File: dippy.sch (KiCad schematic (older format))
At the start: 12 parts, among them J1 Conn_01x02_Female, U1 ATmega328P-PU, U2 RFM95W-915S2, U3 MCP1700-3302E_SOT23, Y1 Crystal_GND2

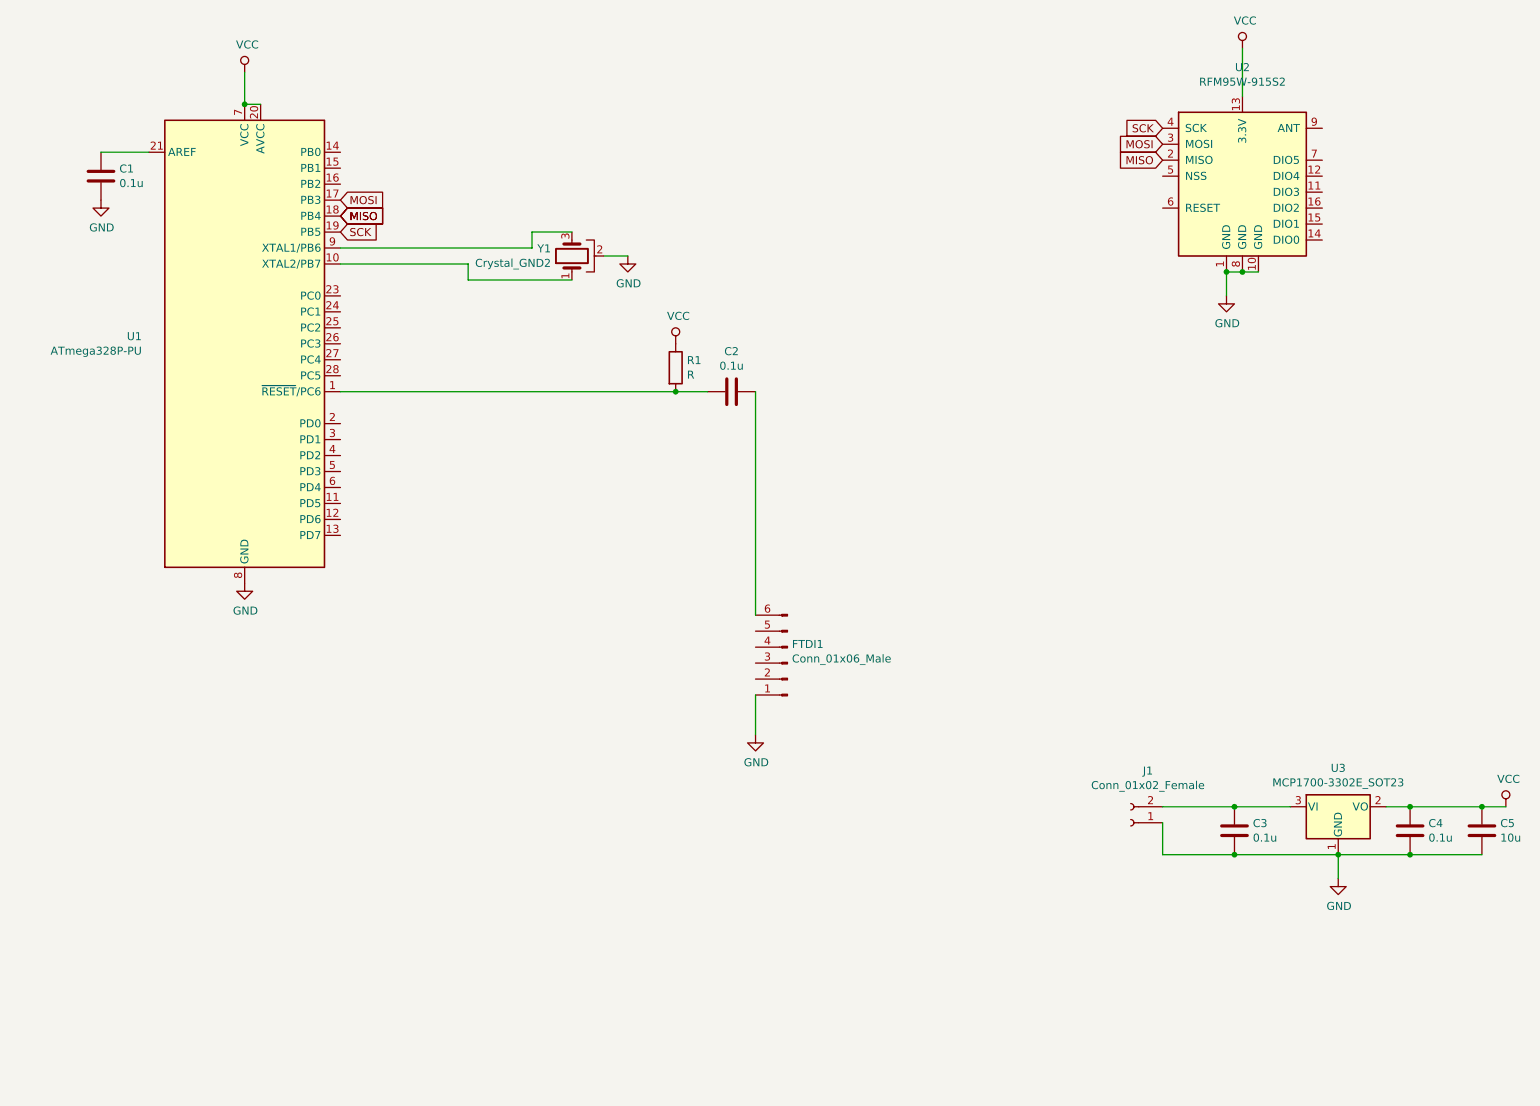
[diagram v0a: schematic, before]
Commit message: update
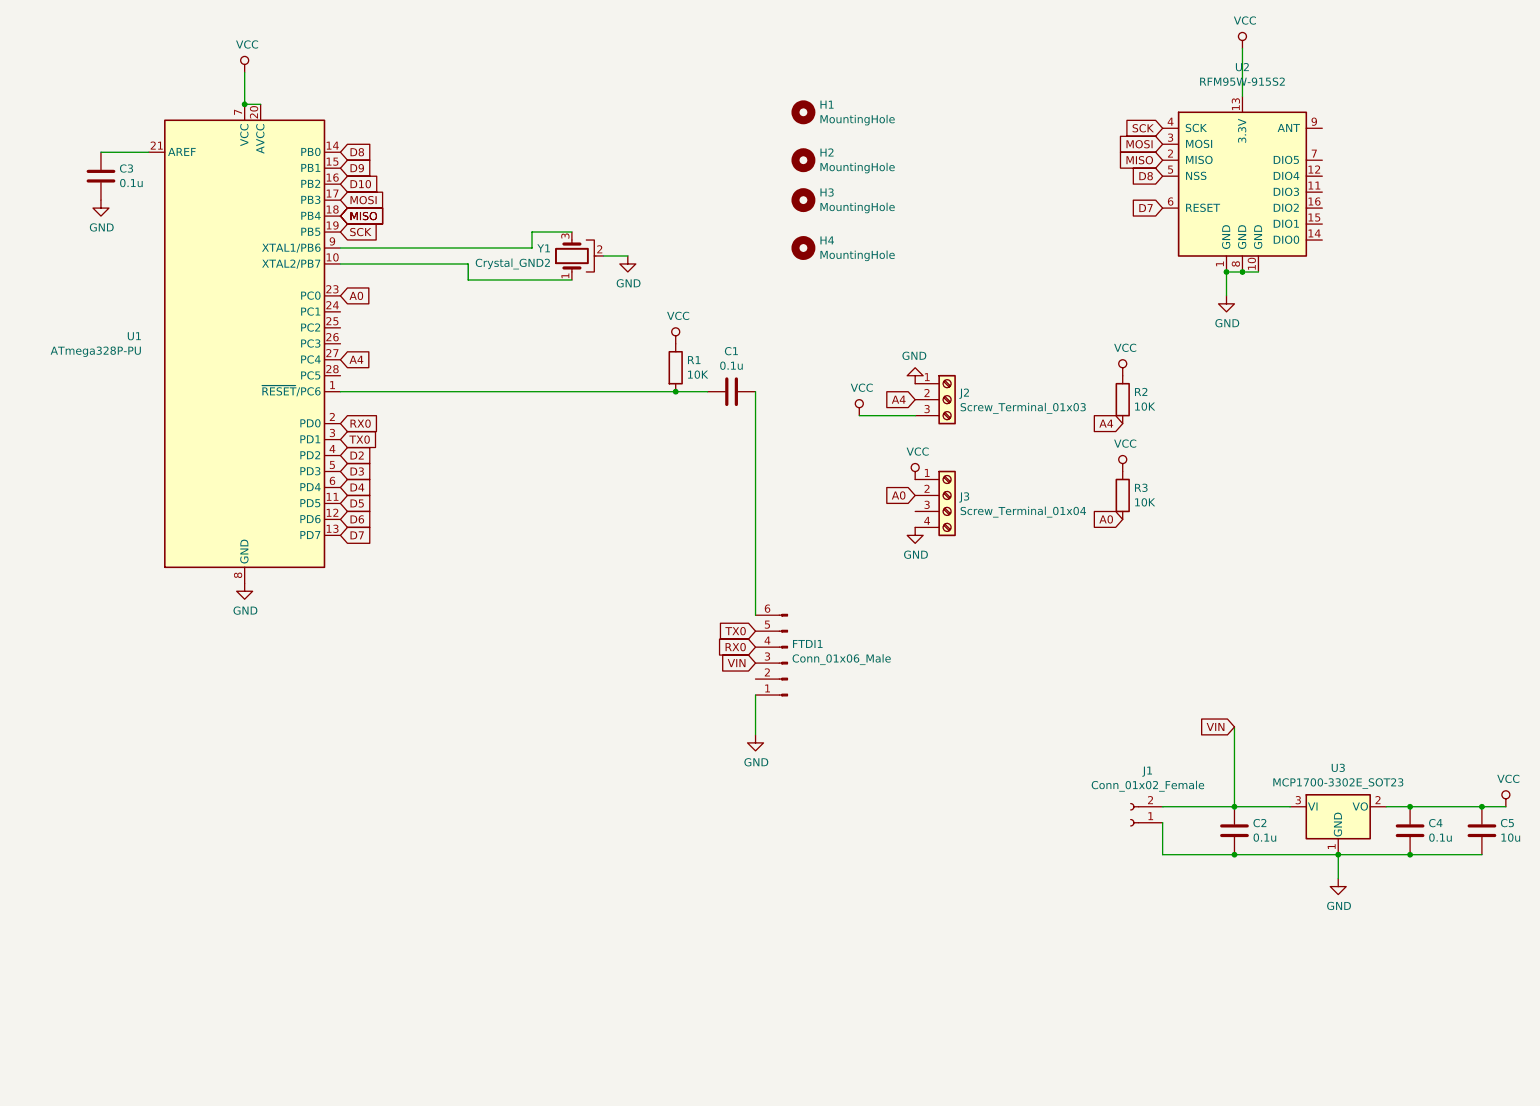
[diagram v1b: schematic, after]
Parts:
- added H1, H2, H3, H4: MountingHole, MountingHole:MountingHole_2.7mm_M2.5, symbol Mechanical:MountingHole
- added J2: Screw_Terminal_01x03, TerminalBlock_Phoenix:TerminalBlock_Phoenix_PT-1,5-3-3.5-H_1x03_P3.50mm_Horizontal, symbol Connector:Screw_Terminal_01x03
- added J3: Screw_Terminal_01x04, TerminalBlock_Phoenix:TerminalBlock_Phoenix_PT-1,5-4-3.5-H_1x04_P3.50mm_Horizontal, symbol Connector:Screw_Terminal_01x04
- added R2, R3: 10K, Resistor_THT:R_Axial_DIN0207_L6.3mm_D2.5mm_P2.54mm_Vertical, symbol Device:R
- C1: renamed from C2; footprint (none) -> Capacitor_THT:C_Disc_D3.0mm_W1.6mm_P2.50mm
- C2: renamed from C3; footprint (none) -> Capacitor_THT:C_Disc_D3.0mm_W1.6mm_P2.50mm
- C3: renamed from C1; footprint (none) -> Capacitor_THT:C_Disc_D3.0mm_W1.6mm_P2.50mm
- C4: footprint (none) -> Capacitor_THT:C_Disc_D3.0mm_W1.6mm_P2.50mm
- C5: footprint (none) -> Capacitor_THT:CP_Radial_D5.0mm_P2.50mm
- FTDI1: footprint (none) -> Connector_PinHeader_2.54mm:PinHeader_1x06_P2.54mm_Horizontal
- J1: footprint (none) -> Connector_PinSocket_2.54mm:PinSocket_1x02_P2.54mm_Vertical
- R1: value R -> 10K; footprint (none) -> Resistor_THT:R_Axial_DIN0207_L6.3mm_D2.5mm_P2.54mm_Vertical
- U3: footprint Package_TO_SOT_SMD:SOT-23 -> Package_TO_SOT_THT:TO-92L_Wide
- Y1: footprint (none) -> Connector_PinSocket_2.54mm:PinSocket_1x03_P2.54mm_Vertical
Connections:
- net GND: now also J2.1 (Pin_1), J3.4 (Pin_4)
- net VCC: now also J2.3 (Pin_3), J3.1 (Pin_1), R2.1, R3.1
- net D5: now reaches U1.11 (PD5)
- net D6: now reaches U1.12 (PD6)
- net D7: now reaches U1.13 (PD7)
- net D7: now also U2.6 (RESET)
- net D8: now reaches U1.14 (PB0)
- net D8: now also U2.5 (NSS)
- net D9: now reaches U1.15 (PB1)
- net D10: now reaches U1.16 (PB2)
- net RX0: now reaches U1.2 (PD0)
- net RX0: now also FTDI1.4 (Pin_4)
- net A0: now reaches U1.23 (PC0)
- net A0: now also J3.2 (Pin_2), R3.2
- net A4: now reaches U1.27 (PC4)
- net A4: now also J2.2 (Pin_2), R2.2
- net TX0: now reaches U1.3 (PD1)
- net TX0: now also FTDI1.5 (Pin_5)
- net D2: now reaches U1.4 (PD2)
- net D3: now reaches U1.5 (PD3)
- net D4: now reaches U1.6 (PD4)
- net VIN: now reaches FTDI1.3 (Pin_3)
- net VIN: now also C2.1, J1.2 (Pin_2), U3.3 (VI)
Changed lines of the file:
@@
 F 0 "Y1" V 4796 2231 50  0000 L CNN
 F 1 "Crystal_GND2" V 4705 2231 50  0000 L CNN
-F 2 "" H 4750 2100 50  0001 C CNN
+F 2 "Connector_PinSocket_2.54mm:PinSocket_1x03_P2.54mm_Vertical" H 4750 2100 50  0001 C CNN
 F 3 "~" H 4750 2100 50  0001 C CNN
 	1    4750 2100
@@
 P 5400 2800
 F 0 "R1" H 5470 2846 50  0000 L CNN
-F 1 "R" H 5470 2755 50  0000 L CNN
-F 2 "" V 5330 2800 50  0001 C CNN
+F 1 "10K" H 5470 2755 50  0000 L CNN
+F 2 "Resistor_THT:R_Axial_DIN0207_L6.3mm_D2.5mm_P2.54mm_Vertical" V 5330 2800 50  0001 C CNN
 F 3 "~" H 5400 2800 50  0001 C CNN
 	1    5400 2800
@@
 $EndComp
 $Comp
-L Device:C C1
+L Device:C C3
 U 1 1 5F266C1D
 P 1800 1600
-F 0 "C1" H 1915 1646 50  0000 L CNN
+F 0 "C3" H 1915 1646 50  0000 L CNN
 F 1 "0.1u" H 1915 1555 50  0000 L CNN
-F 2 "" H 1838 1450 50  0001 C CNN
+F 2 "Capacitor_THT:C_Disc_D3.0mm_W1.6mm_P2.50mm" H 1838 1450 50  0001 C CNN
 F 3 "~" H 1800 1600 50  0001 C CNN
 	1    1800 1600
@@
 $EndComp
 $Comp
-L Device:C C2
+L Device:C C1
 U 1 1 5F26DE4A
 P 5750 2950
-F 0 "C2" V 5498 2950 50  0000 C CNN
+F 0 "C1" V 5498 2950 50  0000 C CNN
 F 1 "0.1u" V 5589 2950 50  0000 C CNN
-F 2 "" H 5788 2800 50  0001 C CNN
+F 2 "Capacitor_THT:C_Disc_D3.0mm_W1.6mm_P2.50mm" H 5788 2800 50  0001 C CNN
 F 3 "~" H 5750 2950 50  0001 C CNN
 	1    5750 2950
@@
 F 0 "U3" H 9550 5792 50  0000 C CNN
 F 1 "MCP1700-3302E_SOT23" H 9550 5701 50  0000 C CNN
-F 2 "Package_TO_SOT_SMD:SOT-23" H 9550 5775 50  0001 C CNN
+F 2 "Package_TO_SOT_THT:TO-92L_Wide" H 9550 5775 50  0001 C CNN
 F 3 "http://ww1.microchip.com/downloads/en/DeviceDoc/20001826D.pdf" H 9550 5550 50  0001 C CNN
 	1    9550 5550
@@
 F 0 "J1" H 8142 5325 50  0000 C CNN
 F 1 "Conn_01x02_Female" H 8142 5416 50  0000 C CNN
-F 2 "" H 8250 5650 50  0001 C CNN
+F 2 "Connector_PinSocket_2.54mm:PinSocket_1x02_P2.54mm_Vertical" H 8250 5650 50  0001 C CNN
 F 3 "~" H 8250 5650 50  0001 C CNN
 	1    8250 5650
@@
 	8450 5650 8450 5850
 $Comp
-L Device:C C3
+L Device:C C2
 U 1 1 5F27AAEF
 P 8900 5700
-F 0 "C3" H 9015 5746 50  0000 L CNN
+F 0 "C2" H 9015 5746 50  0000 L CNN
 F 1 "0.1u" H 9015 5655 50  0000 L CNN
-F 2 "" H 8938 5550 50  0001 C CNN
+F 2 "Capacitor_THT:C_Disc_D3.0mm_W1.6mm_P2.50mm" H 8938 5550 50  0001 C CNN
 F 3 "~" H 8900 5700 50  0001 C CNN
 	1    8900 5700
@@
 F 0 "C4" H 10115 5746 50  0000 L CNN
 F 1 "0.1u" H 10115 5655 50  0000 L CNN
-F 2 "" H 10038 5550 50  0001 C CNN
+F 2 "Capacitor_THT:C_Disc_D3.0mm_W1.6mm_P2.50mm" H 10038 5550 50  0001 C CNN
 F 3 "~" H 10000 5700 50  0001 C CNN
 	1    10000 5700
@@
 F 0 "C5" H 10565 5746 50  0000 L CNN
 F 1 "10u" H 10565 5655 50  0000 L CNN
-F 2 "" H 10488 5550 50  0001 C CNN
+F 2 "Capacitor_THT:CP_Radial_D5.0mm_P2.50mm" H 10488 5550 50  0001 C CNN
 F 3 "~" H 10450 5700 50  0001 C CNN
 	1    10450 5700
@@
 F 0 "FTDI1" H 6072 4532 50  0000 R CNN
 F 1 "Conn_01x06_Male" H 6072 4623 50  0000 R CNN
-F 2 "" H 6100 4650 50  0001 C CNN
+F 2 "Connector_PinHeader_2.54mm:PinHeader_1x06_P2.54mm_Horizontal" H 6100 4650 50  0001 C CNN
 F 3 "~" H 6100 4650 50  0001 C CNN
 	1    6100 4650
@@
 Wire Wire Line
 	3300 2150 4100 2150
+Text GLabel 3300 3450 2    50   Input ~ 0
+D3
+Text GLabel 3300 3550 2    50   Input ~ 0
+D4
+Text GLabel 3300 3650 2    50   Input ~ 0
+D5
+Text GLabel 3300 3750 2    50   Input ~ 0
+D6
+Text GLabel 5900 4650 0    50   Input ~ 0
+VIN
+Text GLabel 5900 4550 0    50   Input ~ 0
+RX0
+Text GLabel 5900 4450 0    50   Input ~ 0
+TX0
+Text GLabel 3300 3150 2    50   Input ~ 0
+RX0
+Text GLabel 3300 3250 2    50   Input ~ 0
+TX0
+Text GLabel 3300 3350 2    50   Input ~ 0
+D2
+Text GLabel 3300 3850 2    50   Input ~ 0
+D7
+Text GLabel 3300 1450 2    50   Input ~ 0
+D8
+Text GLabel 3300 1550 2    50   Input ~ 0
+D9
+Text GLabel 3300 1650 2    50   Input ~ 0
+D10
+Text GLabel 8450 1600 0    50   Input ~ 0
+D8
+Text GLabel 8450 1800 0    50   Input ~ 0
+D7
+$Comp
+L Mechanical:MountingHole H1
+U 1 1 5F2F7F92
+P 6200 1200
+F 0 "H1" H 6300 1246 50  0000 L CNN
+F 1 "MountingHole" H 6300 1155 50  0000 L CNN
+F 2 "MountingHole:MountingHole_2.7mm_M2.5" H 6200 1200 50  0001 C CNN
+F 3 "~" H 6200 1200 50  0001 C CNN
+	1    6200 1200
+	1    0    0    -1
+$EndComp
+$Comp
+L Mechanical:MountingHole H2
+U 1 1 5F2F84A7
+P 6200 1500
+F 0 "H2" H 6300 1546 50  0000 L CNN
+F 1 "MountingHole" H 6300 1455 50  0000 L CNN
+F 2 "MountingHole:MountingHole_2.7mm_M2.5" H 6200 1500 50  0001 C CNN
+F 3 "~" H 6200 1500 50  0001 C CNN
+	1    6200 1500
+	1    0    0    -1
+$EndComp
+$Comp
+L Mechanical:MountingHole H3
+U 1 1 5F30039A
+P 6200 1750
+F 0 "H3" H 6300 1796 50  0000 L CNN
+F 1 "MountingHole" H 6300 1705 50  0000 L CNN
+F 2 "MountingHole:MountingHole_2.7mm_M2.5" H 6200 1750 50  0001 C CNN
+F 3 "~" H 6200 1750 50  0001 C CNN
+	1    6200 1750
+	1    0    0    -1
+$EndComp
+$Comp
+L Mechanical:MountingHole H4
+U 1 1 5F30064C
+P 6200 2050
+F 0 "H4" H 6300 2096 50  0000 L CNN
+F 1 "MountingHole" H 6300 2005 50  0000 L CNN
+F 2 "MountingHole:MountingHole_2.7mm_M2.5" H 6200 2050 50  0001 C CNN
+F 3 "~" H 6200 2050 50  0001 C CNN
+	1    6200 2050
+	1    0    0    -1
+$EndComp
+$Comp
+L Connector:Screw_Terminal_01x03 J2
+U 1 1 5F31163E
+P 7100 3000
+F 0 "J2" H 7180 3042 50  0000 L CNN
+F 1 "Screw_Terminal_01x03" H 7180 2951 50  0000 L CNN
+F 2 "TerminalBlock_Phoenix:TerminalBlock_Phoenix_PT-1,5-3-3.5-H_1x03_P3.50mm_Horizontal" H 7100 3000 50  0001 C CNN
+F 3 "~" H 7100 3000 50  0001 C CNN
+	1    7100 3000
+	1    0    0    -1
+$EndComp
+$Comp
+L Connector:Screw_Terminal_01x04 J3
+U 1 1 5F312484
+P 7100 3600
+F 0 "J3" H 7180 3592 50  0000 L CNN
+F 1 "Screw_Terminal_01x04" H 7180 3501 50  0000 L CNN
+F 2 "TerminalBlock_Phoenix:TerminalBlock_Phoenix_PT-1,5-4-3.5-H_1x04_P3.50mm_Horizontal" H 7100 3600 50  0001 C CNN
+F 3 "~" H 7100 3600 50  0001 C CNN
+	1    7100 3600
+	1    0    0    -1
+$EndComp
+$Comp
+L power:VCC #PWR0111
+U 1 1 5F31DB78
+P 6550 3100
+F 0 "#PWR0111" H 6550 2950 50  0001 C CNN
+F 1 "VCC" H 6567 3273 50  0000 C CNN
+F 2 "" H 6550 3100 50  0001 C CNN
+F 3 "" H 6550 3100 50  0001 C CNN
+	1    6550 3100
+	1    0    0    -1
+$EndComp
+Wire Wire Line
+	6900 3100 6550 3100
+Text GLabel 3300 2750 2    50   Input ~ 0
+A4
+Text GLabel 6900 3000 0    50   Input ~ 0
+A4
+$Comp
+L power:GND #PWR0112
+U 1 1 5F3218C4
+P 6900 2900
+F 0 "#PWR0112" H 6900 2650 50  0001 C CNN
+F 1 "GND" H 6905 2727 50  0000 C CNN
+F 2 "" H 6900 2900 50  0001 C CNN
+F 3 "" H 6900 2900 50  0001 C CNN
+	1    6900 2900
+	-1   0    0    1
+$EndComp
+$Comp
+L Device:R R2
+U 1 1 5F322886
+P 8200 3000
+F 0 "R2" H 8270 3046 50  0000 L CNN
+F 1 "10K" H 8270 2955 50  0000 L CNN
+F 2 "Resistor_THT:R_Axial_DIN0207_L6.3mm_D2.5mm_P2.54mm_Vertical" V 8130 3000 50  0001 C CNN
+F 3 "~" H 8200 3000 50  0001 C CNN
+	1    8200 3000
+	1    0    0    -1
+$EndComp
+$Comp
+L power:VCC #PWR0113
+U 1 1 5F322DF7
+P 8200 2850
+F 0 "#PWR0113" H 8200 2700 50  0001 C CNN
+F 1 "VCC" H 8217 3023 50  0000 C CNN
+F 2 "" H 8200 2850 50  0001 C CNN
+F 3 "" H 8200 2850 50  0001 C CNN
+	1    8200 2850
+	1    0    0    -1
+$EndComp
+Text GLabel 8200 3150 0    50   Input ~ 0
+A4
+$Comp
+L power:VCC #PWR0114
+U 1 1 5F32A308
+P 6900 3500
+F 0 "#PWR0114" H 6900 3350 50  0001 C CNN
+F 1 "VCC" H 6917 3673 50  0000 C CNN
+F 2 "" H 6900 3500 50  0001 C CNN
+F 3 "" H 6900 3500 50  0001 C CNN
+	1    6900 3500
+	1    0    0    -1
+$EndComp
+Text GLabel 3300 2350 2    50   Input ~ 0
+A0
+Text GLabel 6900 3600 0    50   Input ~ 0
+A0
+$Comp
+L Device:R R3
+U 1 1 5F334BCF
+P 8200 3600
+F 0 "R3" H 8270 3646 50  0000 L CNN
+F 1 "10K" H 8270 3555 50  0000 L CNN
+F 2 "Resistor_THT:R_Axial_DIN0207_L6.3mm_D2.5mm_P2.54mm_Vertical" V 8130 3600 50  0001 C CNN
+F 3 "~" H 8200 3600 50  0001 C CNN
+	1    8200 3600
+	1    0    0    -1
+$EndComp
+$Comp
+L power:VCC #PWR0115
+U 1 1 5F3351C9
+P 8200 3450
+F 0 "#PWR0115" H 8200 3300 50  0001 C CNN
+F 1 "VCC" H 8217 3623 50  0000 C CNN
+F 2 "" H 8200 3450 50  0001 C CNN
+F 3 "" H 8200 3450 50  0001 C CNN
+	1    8200 3450
+	1    0    0    -1
+$EndComp
+Text GLabel 8200 3750 0    50   Input ~ 0
+A0
+$Comp
+L power:GND #PWR0116
+U 1 1 5F33656E
+P 6900 3800
+F 0 "#PWR0116" H 6900 3550 50  0001 C CNN
+F 1 "GND" H 6905 3627 50  0000 C CNN
+F 2 "" H 6900 3800 50  0001 C CNN
+F 3 "" H 6900 3800 50  0001 C CNN
+	1    6900 3800
+	1    0    0    -1
+$EndComp
+Text GLabel 8900 5050 0    50   Input ~ 0
+VIN
+Wire Wire Line
+	8900 5050 8900 5550
 $EndSCHEMATC

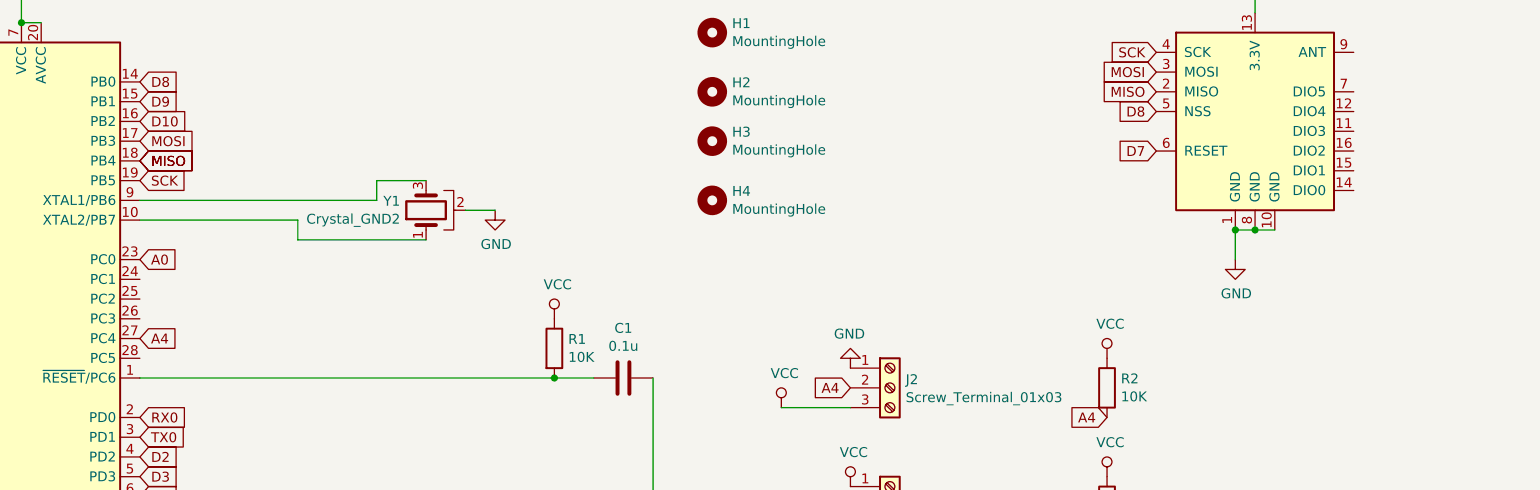
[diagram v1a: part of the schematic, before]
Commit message: update
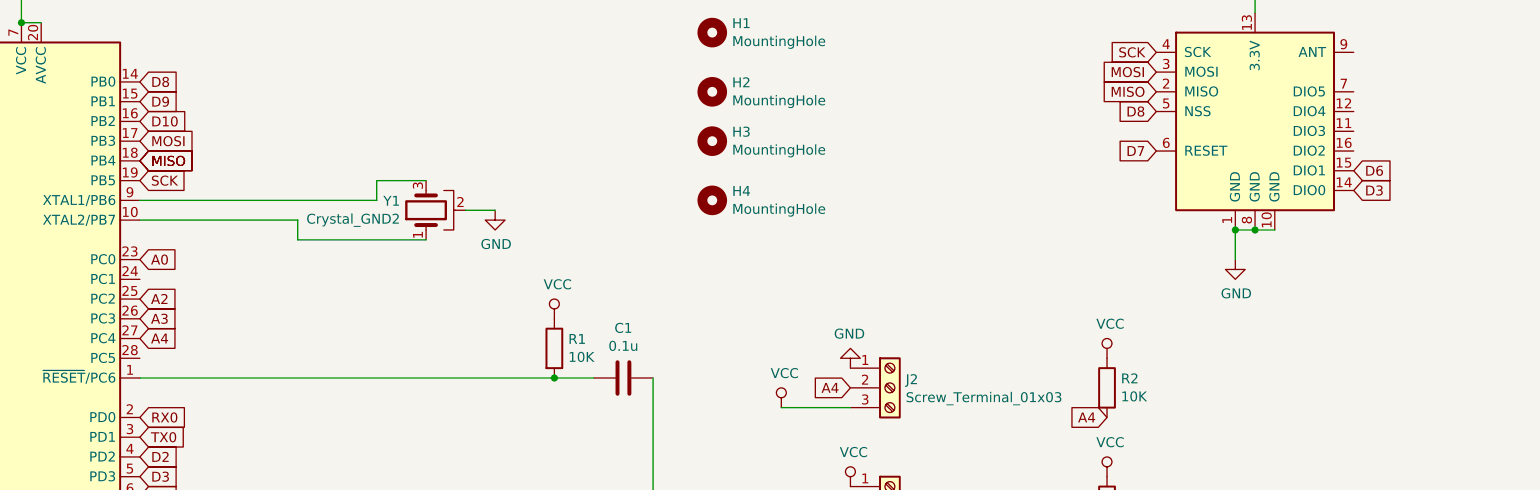
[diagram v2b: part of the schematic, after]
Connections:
- net D3: now also U2.14 (DIO0)
- net D6: now also U2.15 (DIO1)
- net A2: now reaches U1.25 (PC2)
- net A3: now reaches U1.26 (PC3)
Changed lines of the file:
@@
 Wire Wire Line
 	8900 5050 8900 5550
+Text GLabel 3300 2650 2    50   Input ~ 0
+A3
+Text GLabel 3300 2550 2    50   Input ~ 0
+A2
+Text GLabel 9450 1900 2    50   Input ~ 0
+D6
+Text GLabel 9450 2000 2    50   Input ~ 0
+D3
 $EndSCHEMATC
